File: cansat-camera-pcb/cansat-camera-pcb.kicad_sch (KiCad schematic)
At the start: 25 parts, among them SW2 SW_Push, U4 STM32H743ZITx, Y1 24MHz

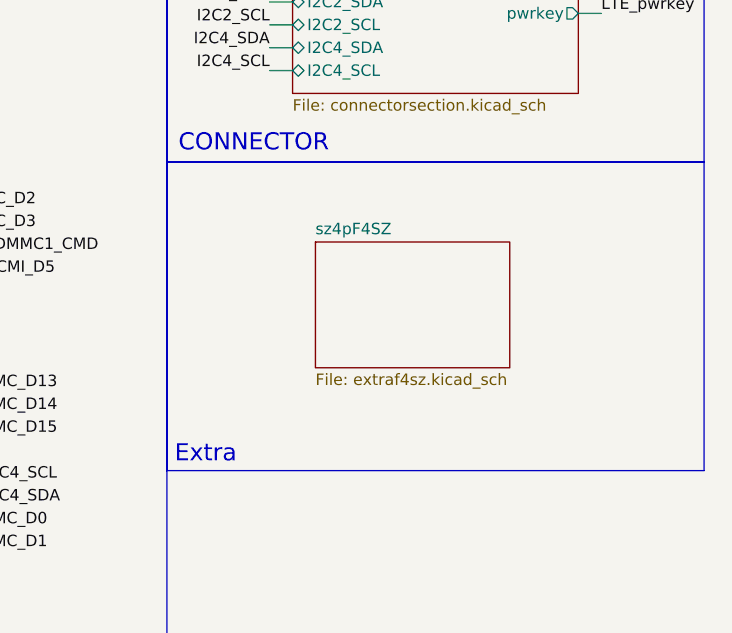
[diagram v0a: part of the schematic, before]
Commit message: Camera_Final
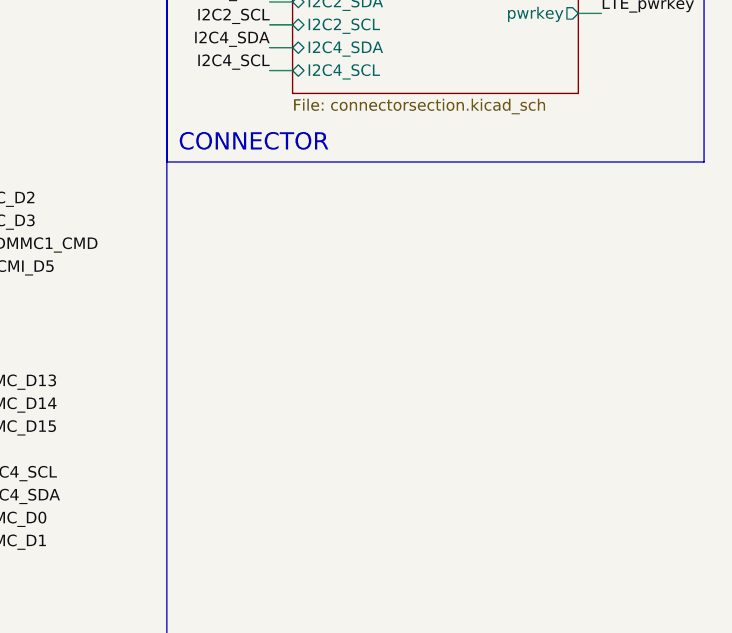
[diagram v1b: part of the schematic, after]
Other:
- removed sheet sz4pF4SZ
- note removed: "Extra"
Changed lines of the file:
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@@
 	)
 	(rectangle
-		(start 144.78 194.31)
-		(end 204.47 228.6)
-		(stroke
-			(width 0)
-			(type default)
-		)
-		(fill
-			(type none)
-		)
-	)
-	(rectangle
 		(start 19.05 17.78)
 		(end 144.78 281.94)
@@
 		)
 	)
-	(text "Extra"
-		(exclude_from_sim no)
-		(at 149.098 226.822 0)
-		(effects
-			(font
-				(size 1.905 1.905)
-			)
-		)
-	)
 	(junction
 		(at 100.33 57.15)
@@
 			)
 		)
-		(instances
-			(project "cansat-camera-pcb"
-				(path "/ff55e53a-9379-43eb-9b08-9bace1f81889"
-					(page "6")
-				)
-			)
-		)
-	)
-	(sheet
-		(at 161.29 203.2)
-		(size 21.59 13.97)
-		(exclude_from_sim no)
-		(in_bom yes)
-		(on_board yes)
-		(dnp no)
-		(fields_autoplaced yes)
-		(stroke
-			(width 0.1524)
-			(type solid)
-		)
-		(fill
-			(color 0 0 0 0.0000)
-		)
-		(property "Sheetname" "sz4pF4SZ"
-			(at 161.29 202.4884 0)
-			(effects
-				(font
-					(size 1.27 1.27)
-				)
-				(justify left bottom)
-			)
-		)
-		(property "Sheetfile" "extraf4sz.kicad_sch"
-			(at 161.29 217.7546 0)
-			(effects
-				(font
-					(size 1.27 1.27)
-				)
-				(justify left top)
-			)
-		)
